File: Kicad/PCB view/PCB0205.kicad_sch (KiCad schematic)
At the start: 18 parts, among them J1 Soil Mositure Sen, SW1 SW_DPST_x2, SW2 SW_Push, SW3 SW_SPDT, U1 MOUDLE-SEEEDUINO-XIAO-ESP32C3, U2 ULN2003, U3 MOUDLE-SEEEDUINO-XIAO-ESP32C3

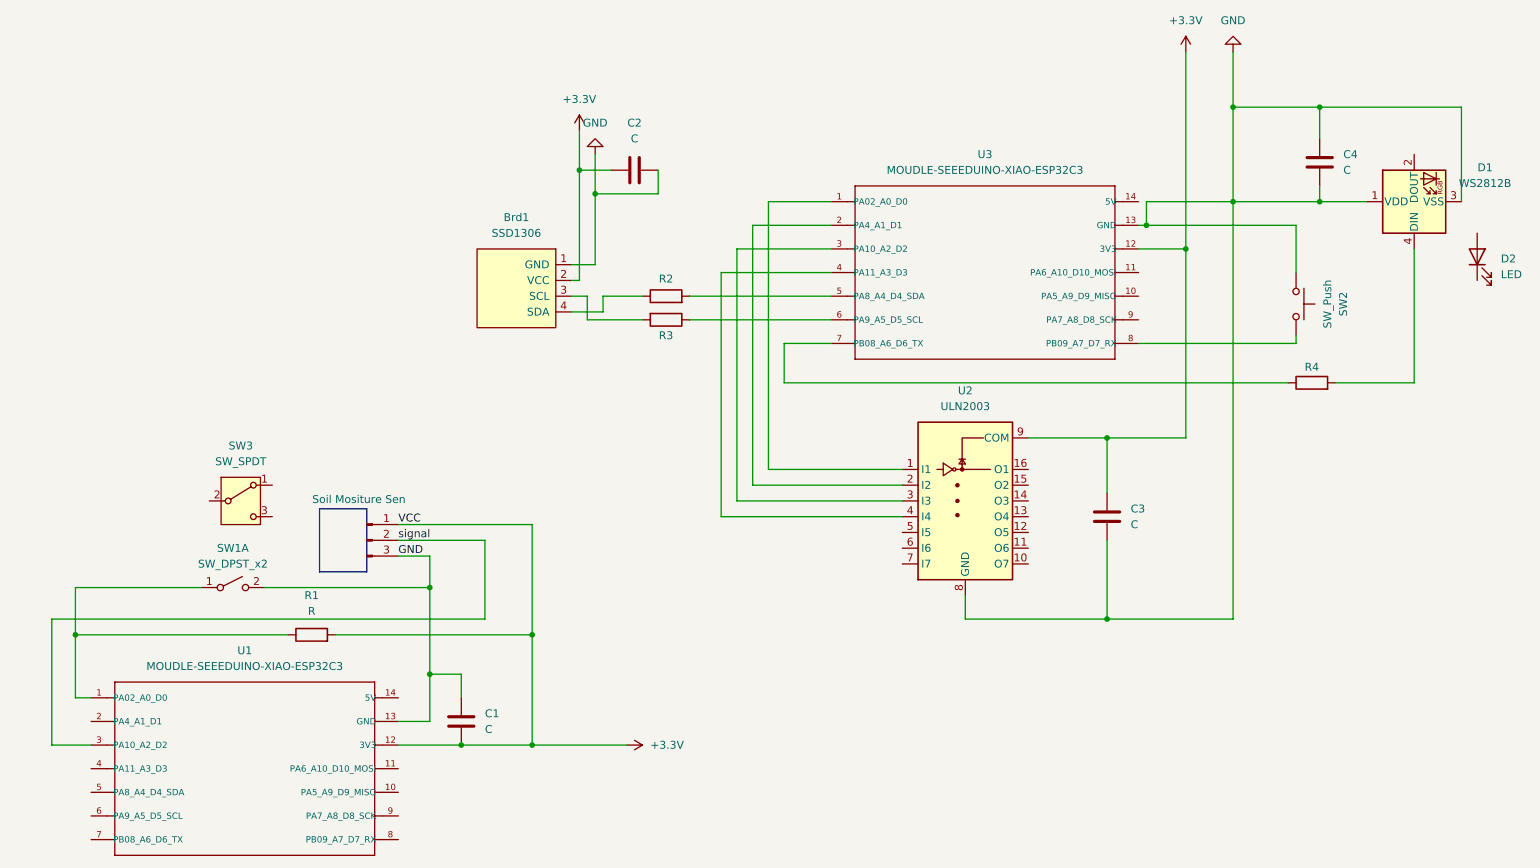
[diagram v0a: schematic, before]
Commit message: Update Soil monitor project files
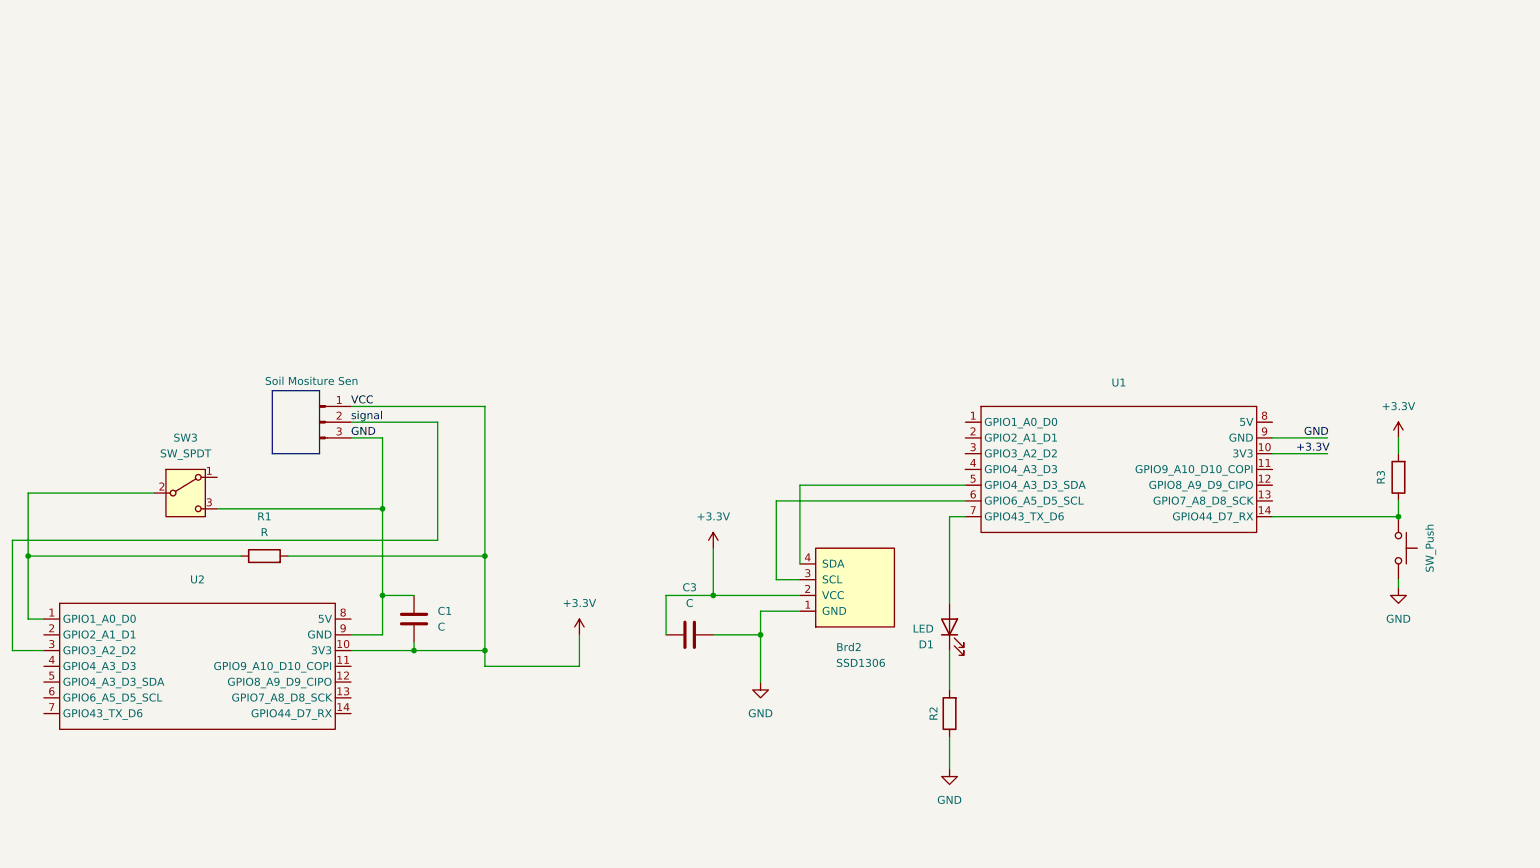
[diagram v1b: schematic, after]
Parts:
- removed Brd1: SSD1306, symbol SSD1306-128x64_OLED:SSD1306
- removed C2, C4: C, symbol Device:C
- removed D1: WS2812B, LED_SMD:LED_WS2812B_PLCC4_5.0x5.0mm_P3.2mm, symbol LED:WS2812B
- removed D2: LED, symbol Device:LED
- removed R4: R, symbol Device:R
- removed SW1: SW_DPST_x2, symbol Switch:SW_DPST_x2
- removed SW2: SW_Push, symbol Switch:SW_Push
- removed U1, U3: MOUDLE-SEEEDUINO-XIAO-ESP32C3, MOUDLE14P-SMD-2.54-21X17.8MM, symbol XIAO_ESP32C3:MOUDLE-SEEEDUINO-XIAO-ESP32C3
- removed U2: ULN2003, symbol Transistor_Array:ULN2003
- added Brd2: SSD1306, SSD1306:128x64OLED, symbol SSD1306-128x64_OLED:SSD1306
- added D1: LED, LED_SMD:LED_0805_2012Metric_Pad1.15x1.40mm_HandSolder, symbol Device:LED
- added SW1: SW_Push, Connector_PinHeader_2.54mm:PinHeader_1x03_P2.54mm_Vertical, symbol Switch:SW_Push
- added U1, U2: ~, 514_KiCAD_Demo:XIAO_ESP32_SENSE, symbol esp32 C3 xiao:XIAO_ESP32_SENSE
- C1, C3: footprint (none) -> Capacitor_SMD:C_0805_2012Metric_Pad1.18x1.45mm_HandSolder
- J1, SW3: footprint (none) -> Connector_PinHeader_2.54mm:PinHeader_1x03_P2.54mm_Vertical
- R1, R2, R3: footprint (none) -> Resistor_SMD:R_0805_2012Metric_Pad1.20x1.40mm_HandSolder
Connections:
- net +3.3V: now also C3.2, R3.2, Brd2.2 (VCC), U1.10 (3V3), U2.10 (3V3); no longer C3.1
- net GND: now also C3.1, R2.1, SW3.3 (C), Brd2.1 (GND), SW1.2, U1.9 (GND), U2.9 (GND); no longer C3.2
- net signal: now also U2.3 (GPIO3_A2_D2)
- net at R2.2: now also D1.1 (K)
- net at SW3.2 (B): now also R1.1, U2.1 (GPIO1_A0_D0)
- net at R3.1: now also SW1.1, U1.14 (GPIO44_D7_RX)
- new net: D1.2 (A), U1.7 (GPIO43_TX_D6)
- new net: Brd2.4 (SDA), U1.5 (GPIO4_A3_D3_SDA)
- new net: Brd2.3 (SCL), U1.6 (GPIO6_A5_D5_SCL)
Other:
- moved on the sheet: C1, R1, SW3
